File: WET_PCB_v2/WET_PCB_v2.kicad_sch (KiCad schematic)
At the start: 28 parts, among them J10 Conn_01x09_Pin, J11 Conn_01x09_Pin, J2 Conn_01x09_Pin, J3 Conn_01x09_Pin, J4 Pluggable terminal block, J5 Barrel jack, J6 Pluggable Terminal Block, J7 Pluggable Terminal Block, J8 Jumper, U3 Opamp_Quad

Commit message: didnt watch the lecture but made progress ig
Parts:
- added J16: POGO1, Connector_PinHeader_1.00mm:PinHeader_1x01_P1.00mm_Vertical, symbol Connector:Conn_01x01_Pin
- added J21: POGO2, Connector_PinHeader_1.00mm:PinHeader_1x01_P1.00mm_Vertical, symbol Connector:Conn_01x01_Pin
- added R43: R0, Resistor_SMD:R_0805_2012Metric_Pad1.20x1.40mm_HandSolder, symbol Device:R
- J4: value Pluggable terminal block -> Power input
- J6: value Pluggable Terminal Block -> Coil plug
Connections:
- net VPP: no longer R37.1, R7.1
- net currsense_DCDC/Shunt_to_load: now also R43.2
- net DCDC/Vin_DCDC+ renamed DCDC/currsense_FET_side
- net DCDC/currsense_FET_side: now also R43.1
- new net: J16.1 (Pin_1), U7.19 (POGO_PRG)
- new net: J21.1 (Pin_1), U7.20 (POGO_PRG)
- new net DCDC/currsense_cap_side: R37.1, R7.1
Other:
- sheet DCDC ports: added currsense_FET_side, currsense_cap_side; removed none

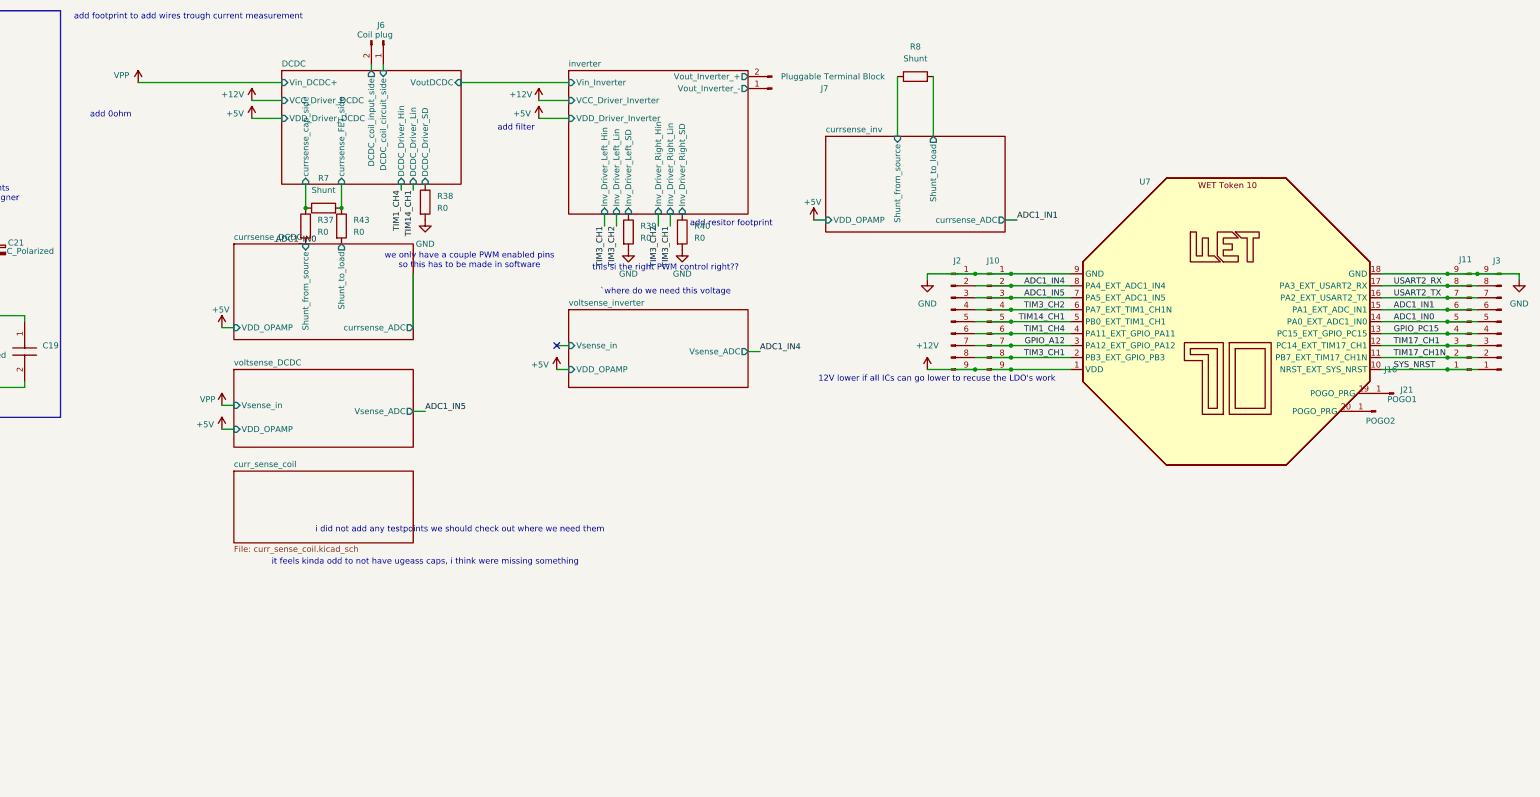
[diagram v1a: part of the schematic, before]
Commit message: i think it fits holy
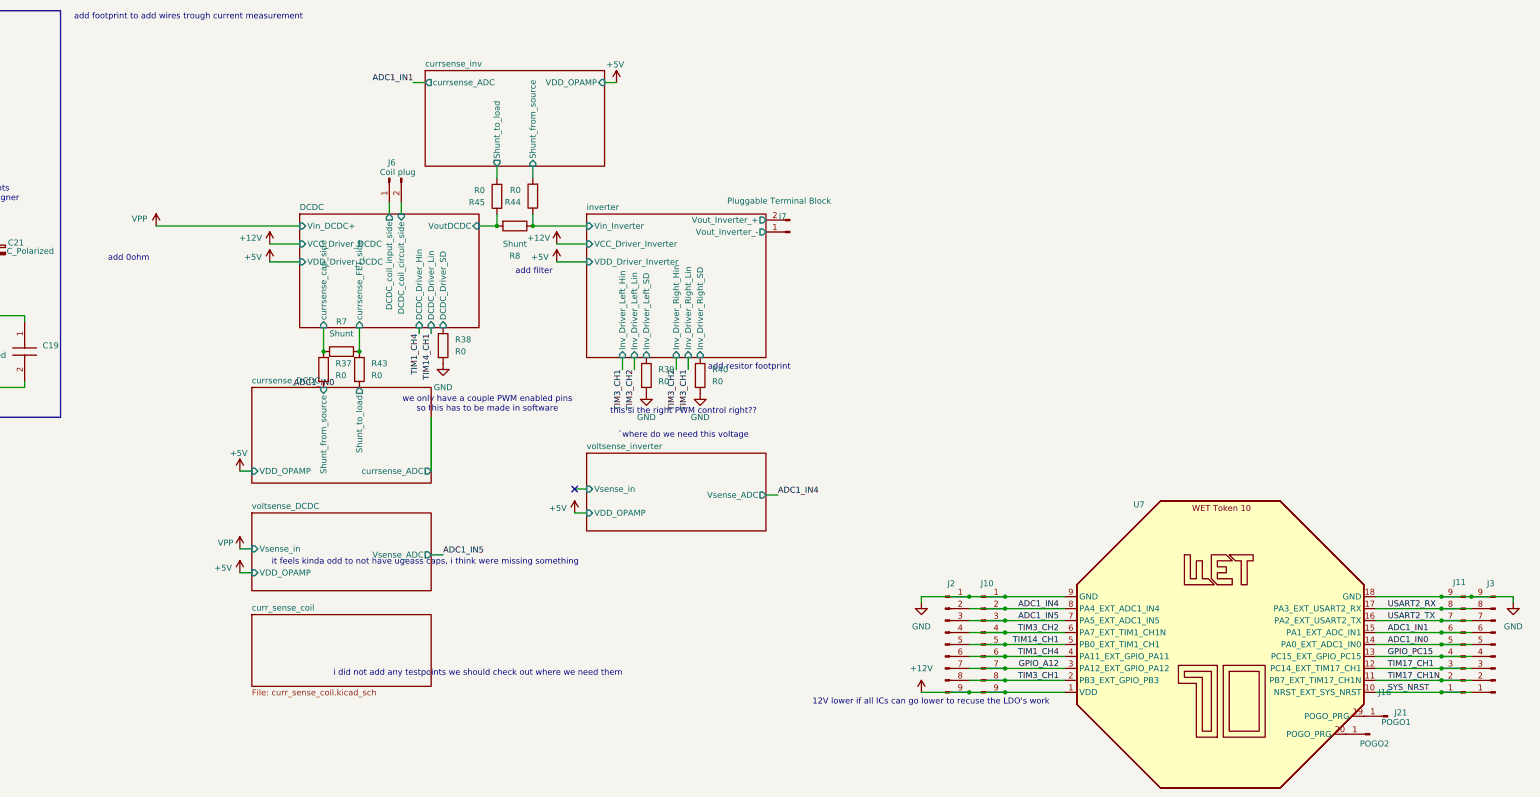
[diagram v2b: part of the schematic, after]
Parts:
- added R44, R45: R0, Resistor_SMD:R_0805_2012Metric_Pad1.20x1.40mm_HandSolder, symbol Device:R
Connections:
- net DCDC/DCDC_coil_circuit_side: now also J6.2 (Pin_2); no longer J6.1 (Pin_1)
- net DCDC/DCDC_coil_input_side: now also J6.1 (Pin_1); no longer J6.2 (Pin_2)
- net DCDC/VoutDCDC: now also R8.2, R45.1
- net currsense_inv/Shunt_from_source: now also R44.2; no longer R8.1
- net currsense_inv/Shunt_to_load: now also R45.2; no longer R8.2
- new net inverter/Vin_Inverter: R44.1, R8.1
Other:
- moved on the sheet: J10, J11, J16, J2, J21, J3, J6, J7, R37, R38, R39, R40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

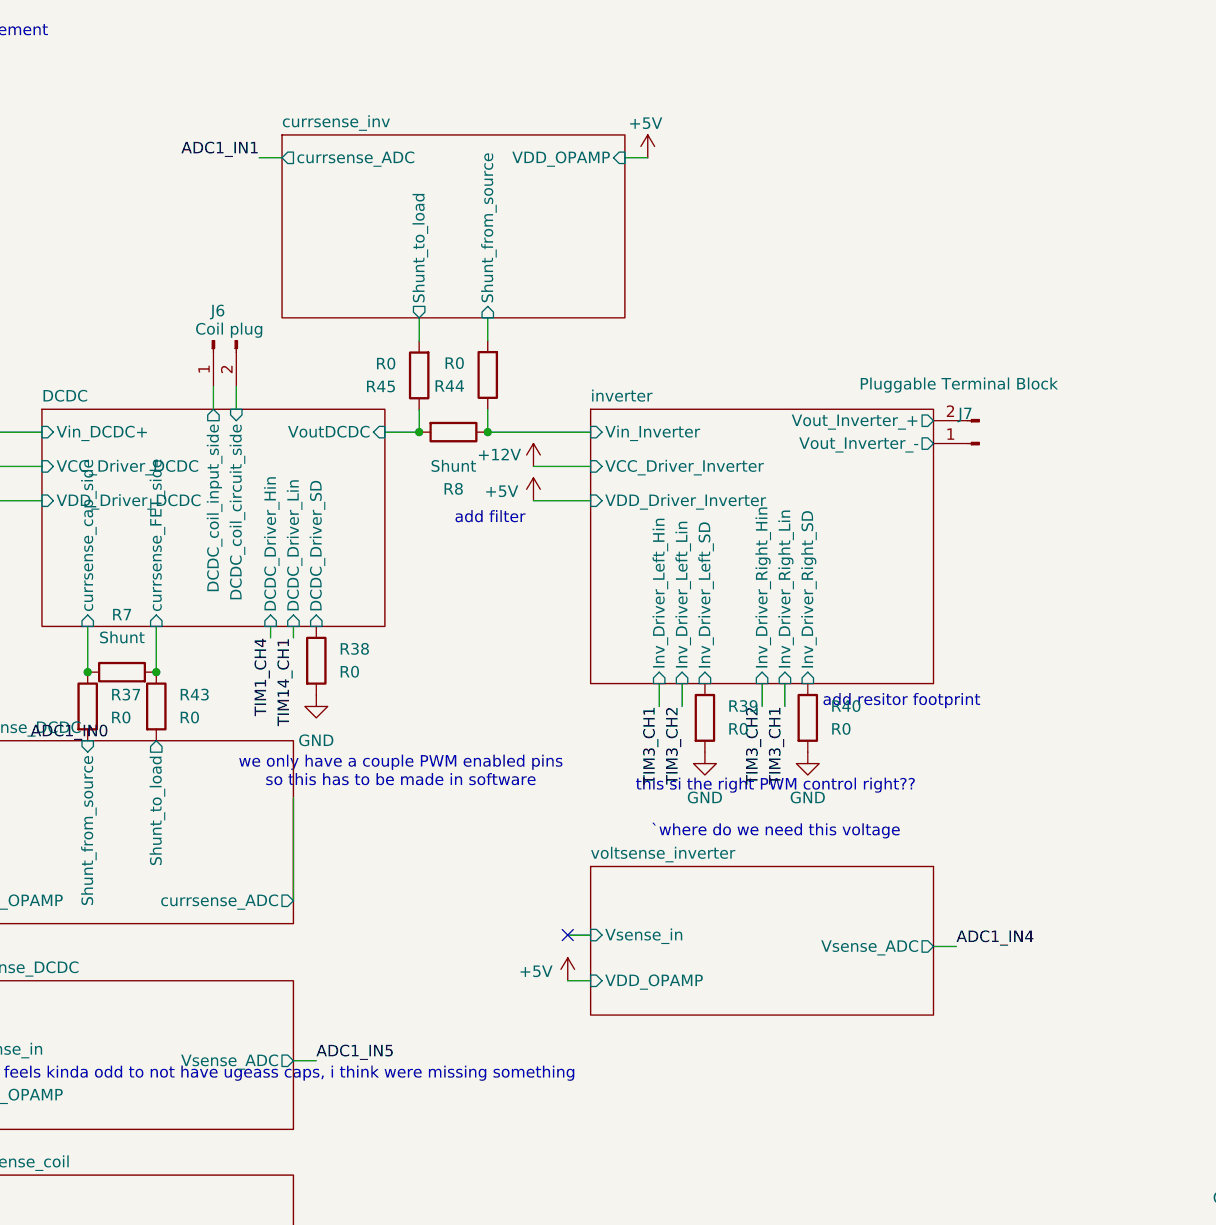
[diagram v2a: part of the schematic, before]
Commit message: lecture done
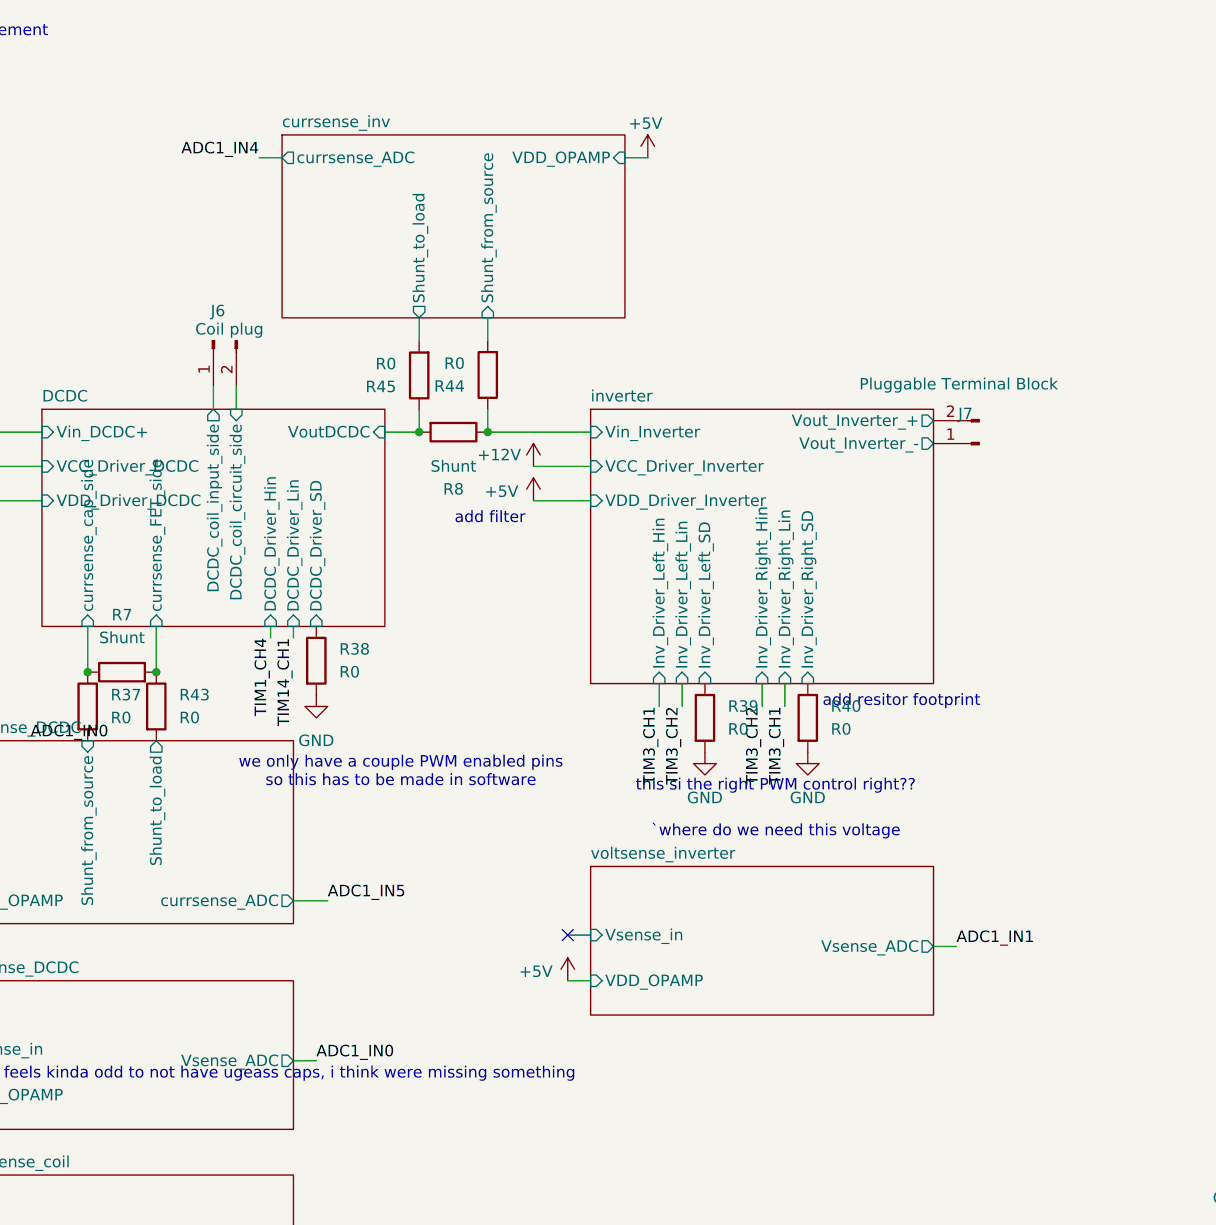
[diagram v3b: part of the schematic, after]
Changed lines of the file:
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@@
 	(wire
 		(pts
+			(xy 172.72 110.49) (xy 176.53 110.49)
+		)
+		(stroke
+			(width 0)
+			(type default)
+		)
+	)
+	(wire
+		(pts
 			(xy 246.38 115.57) (xy 243.84 115.57)
 		)
@@
 	(wire
 		(pts
-			(xy 172.72 99.06) (xy 172.72 110.49)
-		)
-		(stroke
-			(width 0)
-			(type default)
-		)
-	)
-	(wire
-		(pts
 			(xy 49.53 57.15) (xy 62.23 57.15)
 		)
@@
 		)
 	)
+	(label "ADC1_IN5"
+		(at 176.53 110.49 0)
+		(effects
+			(font
+				(size 1.27 1.27)
+			)
+			(justify left bottom)
+		)
+	)
 	(label "TIM3_CH1"
 		(at 213.36 88.9 270)
@@
 		)
 	)
+	(label "ADC1_IN4"
+		(at 168.91 27.94 180)
+		(effects
+			(font
+				(size 1.27 1.27)
+			)
+			(justify right bottom)
+		)
+	)
 	(label "TIM3_CH2"
 		(at 224.79 88.9 270)
@@
 	)
 	(label "ADC1_IN5"
-		(at 175.26 128.27 0)
-		(effects
-			(font
-				(size 1.27 1.27)
-			)
-			(justify left bottom)
-		)
-	)
-	(label "ADC1_IN5"
 		(at 306.07 142.24 180)
 		(effects
@@
 		)
 	)
-	(label "ADC1_IN4"
+	(label "ADC1_IN0"
+		(at 175.26 128.27 0)
+		(effects
+			(font
+				(size 1.27 1.27)
+			)
+			(justify left bottom)
+		)
+	)
+	(label "ADC1_IN1"
 		(at 246.38 115.57 0)
 		(effects
@@
 		)
 	)
-	(label "ADC1_IN1"
-		(at 168.91 27.94 180)
-		(effects
-			(font
-				(size 1.27 1.27)
-			)
-			(justify right bottom)
-		)
-	)
 	(label "TIM1_CH4"
 		(at 31.75 106.68 0)
@@
 	)
 	(group ""
-		(members "a17383a4-d27f-4c25-9e0c-b0df1856b8d8" "b0cb1397-fac0-444b-95f5-30e95b8f9aaf"
-			"e547f70c-7bec-4117-9e0a-e594b69335eb"
-		)
+		(members "a17383a4-d27f-4c25-9e0c-b0df1856b8d8" "e547f70c-7bec-4117-9e0a-e594b69335eb")
 	)
 	(sheet
